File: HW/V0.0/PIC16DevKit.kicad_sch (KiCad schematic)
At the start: 0 parts

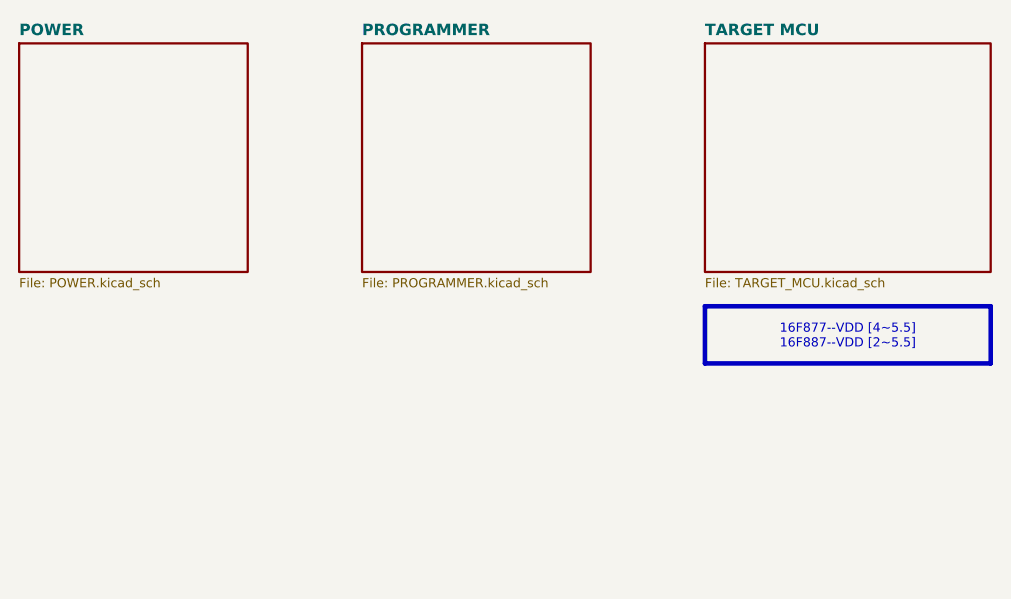
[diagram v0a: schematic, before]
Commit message: PIC16-DevKit-SCH-877 schematic update 5
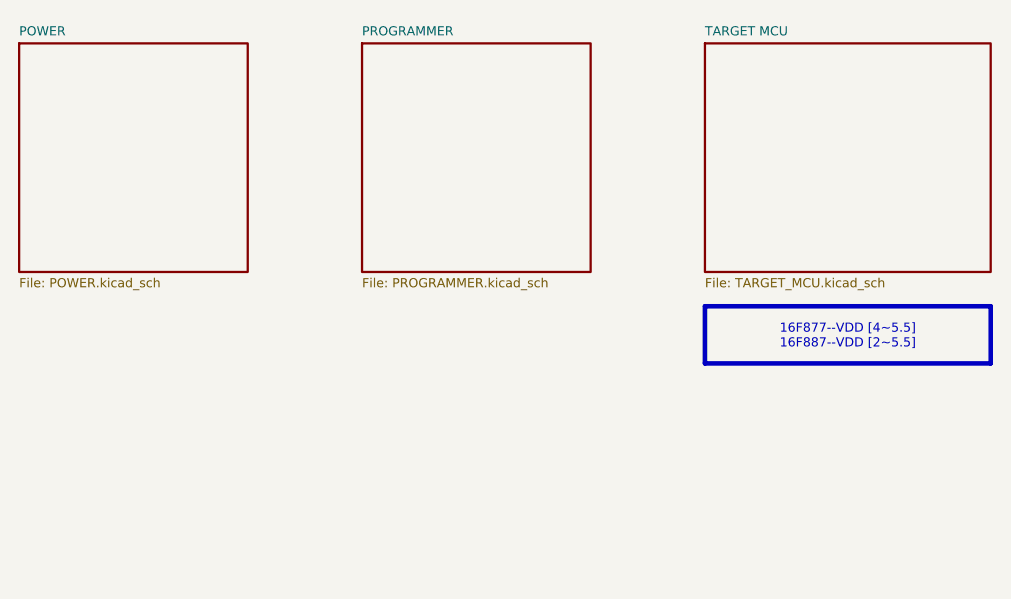
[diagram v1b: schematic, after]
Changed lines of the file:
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@@
 				(font
 					(face "Consolas")
-					(size 1.27 1.27)
-					(bold yes)
+					(size 1.016 1.016)
 				)
 				(justify left bottom)
@@
 				(font
 					(face "Consolas")
-					(size 1.27 1.27)
-					(bold yes)
+					(size 1.016 1.016)
 				)
 				(justify left bottom)
@@
 				(font
 					(face "Consolas")
-					(size 1.27 1.27)
-					(bold yes)
+					(size 1.016 1.016)
 				)
 				(justify left bottom)

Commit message: PIC16-DevKit-SCH-877 schematic update 6
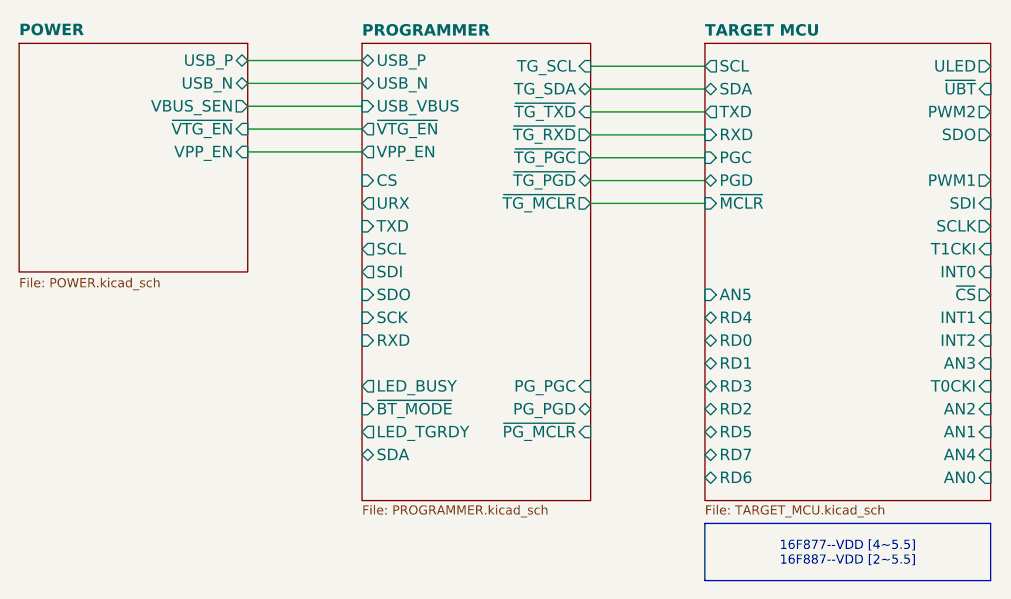
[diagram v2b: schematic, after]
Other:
- sheet POWER ports: added USB_N, USB_P, VBUS_SEN, VPP_EN, ~{VTG_EN}; removed none
- sheet PROGRAMMER ports: added CS, LED_BUSY, LED_TGRDY, PG_PGC, PG_PGD, RXD, SCK, SCL, SDA, SDI, SDO, TG_SCL, TG_SDA, TXD, URX, USB_N, USB_P, USB_VBUS, VPP_EN, ~{BT_MODE}, ~{PG_MCLR}, ~{TG_MCLR}, ~{TG_PGC}, ~{TG_PGD}, ~{TG_RXD}, ~{TG_TXD}, ~{VTG_EN}; removed none
- sheet TARGET MCU ports: added AN0, AN1, AN2, AN3, AN4, AN5, INT0, INT1, INT2, PGC, PGD, PWM1, PWM2, RD0, RD1, RD2, RD3, RD4, RD5, RD6, RD7, RXD, SCL, SCLK, SDA, SDI, SDO, T0CKI, T1CKI, TXD, ULED, ~{CS}, ~{MCLR}, ~{UBT}; removed none
